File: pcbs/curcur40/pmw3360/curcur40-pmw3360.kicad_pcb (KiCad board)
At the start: 2 copper layers, 23.5 x 33 mm, 20 parts, among them J1 Conn_01x08, U1 PMW3360DM-T2QU, U2 TLV74318PDBVR

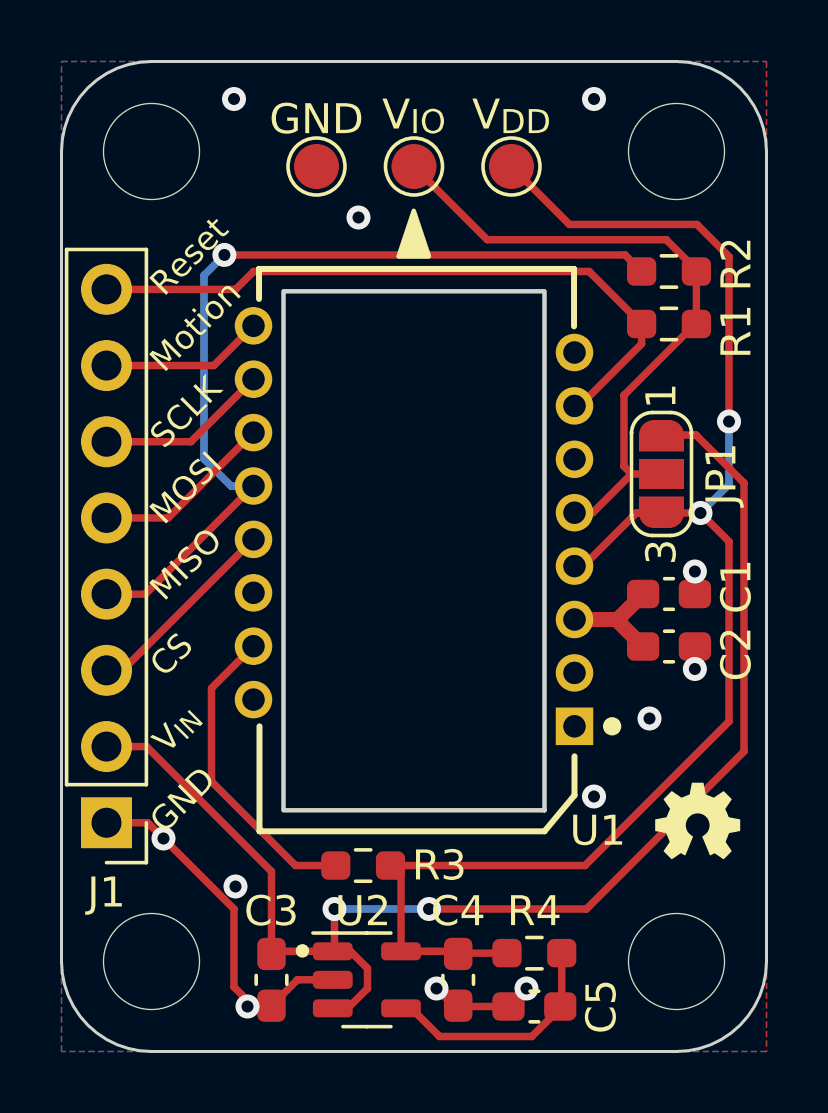
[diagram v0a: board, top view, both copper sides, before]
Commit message: fix trackball-cup
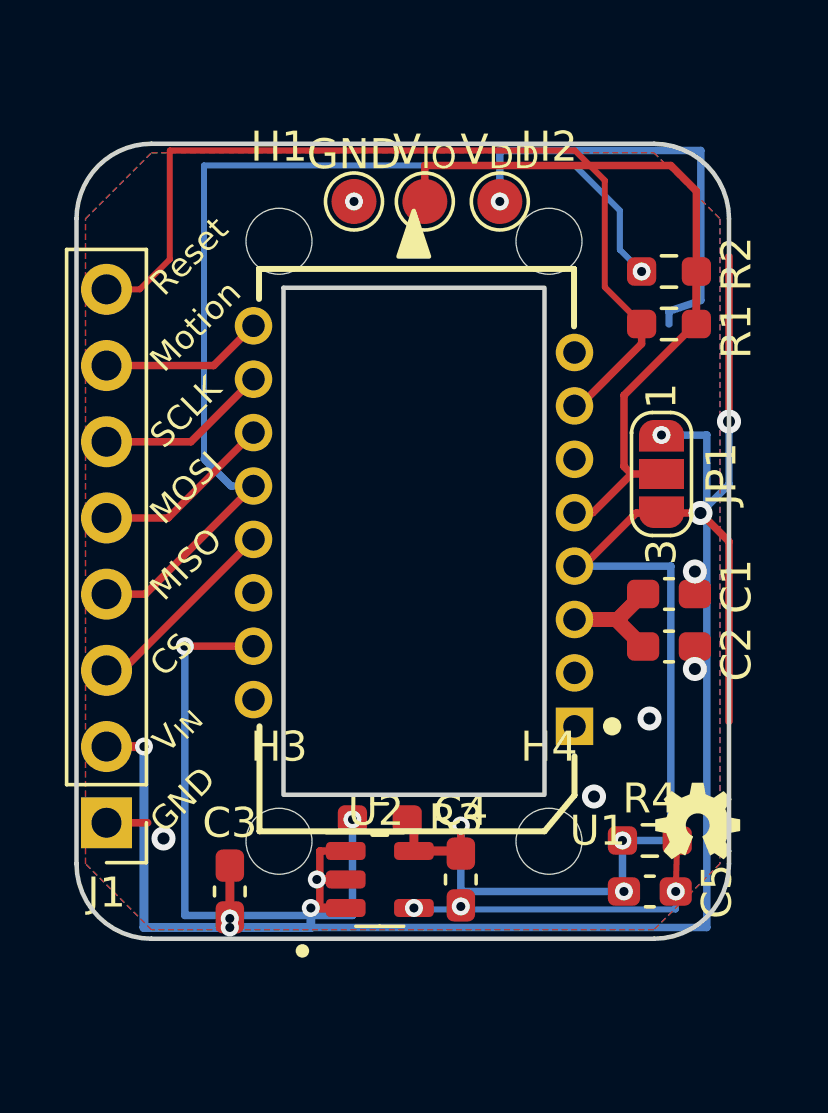
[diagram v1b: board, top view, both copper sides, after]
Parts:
- H1, H2, H3, H4: value MountingHole_Pad -> MountingHole_2.2mm_M2; footprint MountingHole:MountingHole_3.2mm_M3_ISO14580 -> MountingHole_2.2mm_M2
- moved H2 27.4 mm to (150.1, 82.5)
- moved H3 26.5 mm to (141.1, 102.5)
- moved H4 5.84 mm to (150.1, 102.5)
- moved C5 5.43 mm to (153.5, 104.2)
- moved R4 5.38 mm to (153.5, 102.5)
- moved H1 5.20 mm to (141.1, 82.5)
- moved U2 3.37 mm to (144.5, 103.8)
- moved C4 3.35 mm to (147.2, 103.8)
- moved C3 3.26 mm to (139.5, 104.2)
- moved TP3 1.71 mm to (143.6, 81.2)
- moved R3 1.63 mm to (144.5, 101.8)
- moved TP2 1.23 mm to (148.5, 81.2)
- moved TP1 1.22 mm to (146.0, 81.2)
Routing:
- net VDD: track 49.4 -> 63.2 mm, vias 2 -> 5
- net GND: track 15.4 -> 2.34 mm, vias 12 -> 10
- net Net-(U1-LED_P): track 10.4 -> 20.1 mm, vias 0 -> 2
- net /RESET: track 22.6 -> 30.1 mm
- net V_{IN}: track 45.2 -> 51.5 mm, vias 2 -> 4
- net /MISO: track 29.6 -> 35.0 mm
- net V_{IO}: track 22.2 -> 26.4 mm
- net Net-(U2-NC): track 7.94 -> 11.1 mm, vias 0 -> 2
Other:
- board size 23.5 x 33 mm -> 21.8 x 26.5 mm
